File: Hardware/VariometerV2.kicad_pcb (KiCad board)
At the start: 4 copper layers, 107 parts, among them IC1 TP4056, IC2 DW01A-G, IC3 ESP32-S3-WROOM-1, J1 LED_CHRG, J2 LED_STBY, J3 TFT_LCD_CONNECTOR, J4 Conn_01x02_Male, J5 SWD, J6 USB3135-30-A, J7 5-1814832-1, J8 Conn_02x01, J9 MEM2075-00-140-01-A, Q1 AO3400A, Q10 AO3400A, Q2 AO3400A, Q3 AO3401A, Q4 AO3400A, Q5 AO3401A, Q6 AO3400A, Q7 AO3401A, Q8 AO3400A, Q9 AO3401A, SW1 SW_Push, SW2 Switch_SW_Push, SW3 Switch_SW_Push, SW4 SW_Push, U1 TPS76801QDR, U2 SRV05-4, U4 ATGM336H-5N31, U5 SRV05-4, U6 SRV05-4, U7 BMI088, U8 MS5611-01BA

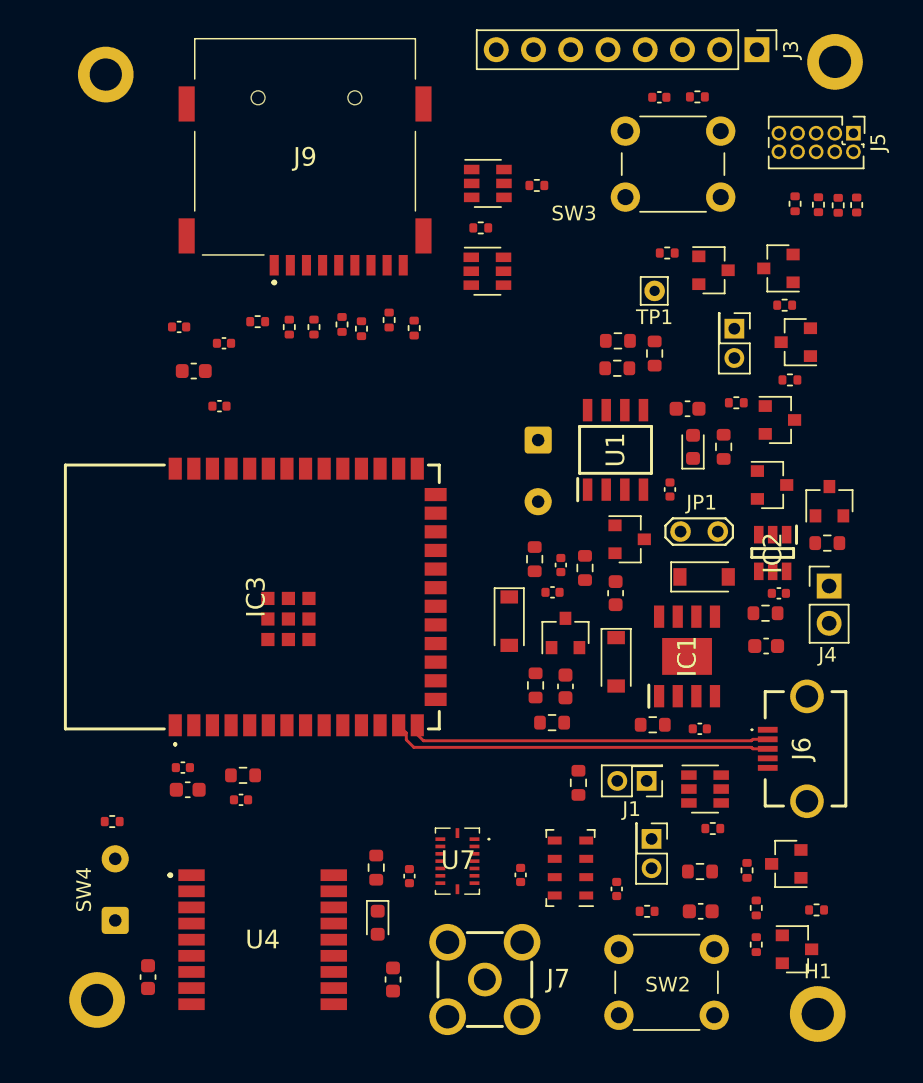
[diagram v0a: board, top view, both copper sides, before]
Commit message: update
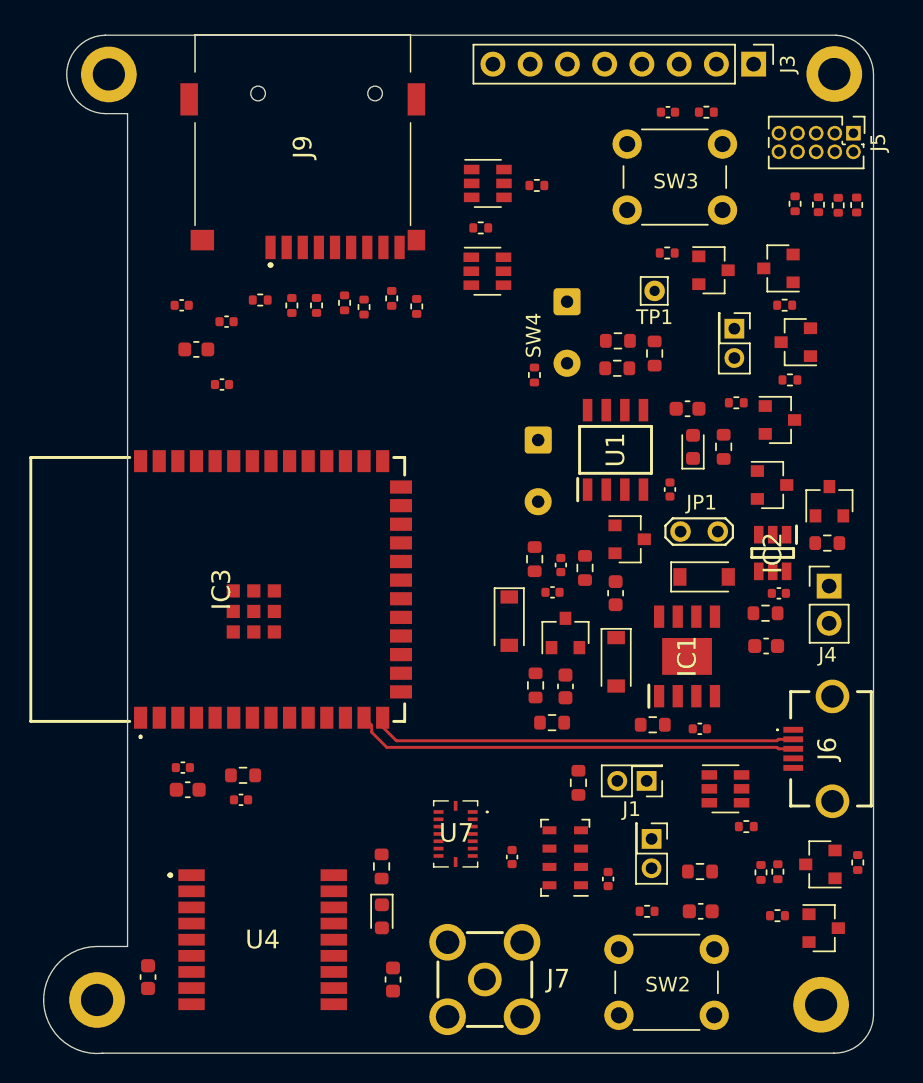
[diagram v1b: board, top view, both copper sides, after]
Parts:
- removed C19: 100nF, Capacitor_SMD:C_0402_1005Metric
- J9: value MEM2075-00-140-01-A -> TFP09-2-12B; footprint Hardware:MEM20750014001A -> Hardware:TFP09212B
- moved SW4 52.3 mm to (56.5, 36.2), turned to 270 degrees
- moved R19 41.9 mm to (54.3, 41.2), turned to 90 degrees
- moved J9 7.99 mm to (38.5, 18.0), turned to 270 degrees
- moved R13 4.28 mm to (76.4, 74.5), turned to 90 degrees
- moved R16 2.45 mm to (70.9, 78.1), turned to 0 degrees
- moved R15 2.44 mm to (69.8, 75.1), turned to 270 degrees
- moved IC3 2.42 mm to (32.7, 55.8)
- moved Q5 2.32 mm to (73.8, 74.6)
- moved Q6 2.32 mm to (74.0, 78.9)
- moved R24 2.29 mm to (68.8, 72.0)
- moved R14 2.10 mm to (70.9, 75.1)
- moved U7 1.86 mm to (49.0, 72.5)
- moved J6 1.74 mm to (74.5, 66.7)
- moved C17 1.49 mm to (33.3, 37.6)
- moved R30 1.49 mm to (35.6, 36.1)
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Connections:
- IC2 pad 4: (no net) -> Net-(IC2-Pad4)
- IC3 pad 15: (no net) -> Net-(IC3-Pad15)
- IC3 pad 16: (no net) -> Net-(IC3-Pad16)
- IC3 pad 36: (no net) -> Net-(IC3-Pad36)
- IC3 pad 37: (no net) -> Net-(IC3-Pad37)
- IC3 pad 5: (no net) -> Net-(IC3-Pad5)
- J5 pad 10: (no net) -> Net-(J5-Pad10)
- J5 pad 7: (no net) -> Net-(J5-Pad7)
- J6 pad 4: (no net) -> Net-(J6-Pad4)
- R30 pad 2: Net-(J9-PadP1) -> Net-(J9-Pad1)
- R34 pad 2: Net-(J9-PadP8) -> Net-(J9-Pad8)
- R35 pad 2: Net-(J9-PadP5) -> Net-(J9-Pad5)
- U1 pad 8: (no net) -> Net-(U1-Pad8)
- U2 pad 4: (no net) -> Net-(U2-Pad4)
- U2 pad 6: (no net) -> Net-(U2-Pad6)
- U4 pad 13: (no net) -> Net-(U4-Pad13)
- U4 pad 15: (no net) -> Net-(U4-Pad15)
- U4 pad 16: (no net) -> Net-(U4-Pad16)
- U4 pad 17: (no net) -> Net-(U4-Pad17)
- U4 pad 18: (no net) -> Net-(U4-Pad18)
- U4 pad 7: (no net) -> Net-(U4-Pad7)
- U4 pad 9: (no net) -> Net-(U4-Pad9)
- U5 pad 3: Net-(J9-PadP1) -> Net-(J9-Pad1)
- U5 pad 6: Net-(J9-PadP5) -> Net-(J9-Pad5)
- U6 pad 3: Net-(J9-PadP8) -> Net-(J9-Pad8)
- U7 pad 1: (no net) -> Net-(U7-Pad1)
- U7 pad 13: (no net) -> Net-(U7-Pad13)
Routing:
- net USB_D-: track 26.1 -> 30.4 mm
- net USB_D+: track 24.8 -> 29.1 mm
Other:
- board outline added: 56.6 x 69.4 mm
